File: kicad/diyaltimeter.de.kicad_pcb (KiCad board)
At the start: 2 copper layers, 45.7 x 97.8 mm, 12 parts, among them J1 Buttons, J2 Display, J3 links, J4 rechts, J5 I2C_BMP280, J6 I2C_BMP280_2, J7 RTC DS3231, J8 Conn_01x04_Male, SW1 SW_Push, SW2 SW_Push, SW3 SW_Push

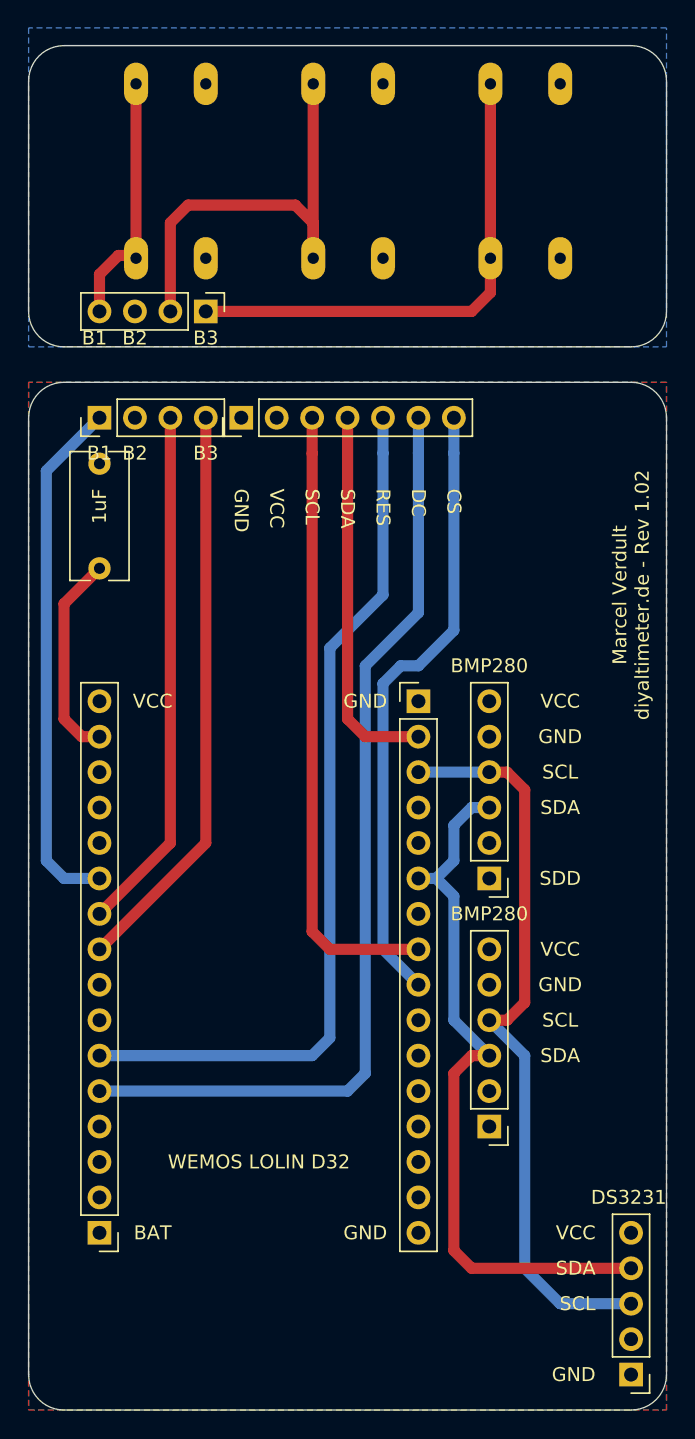
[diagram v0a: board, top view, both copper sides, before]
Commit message: final pcb
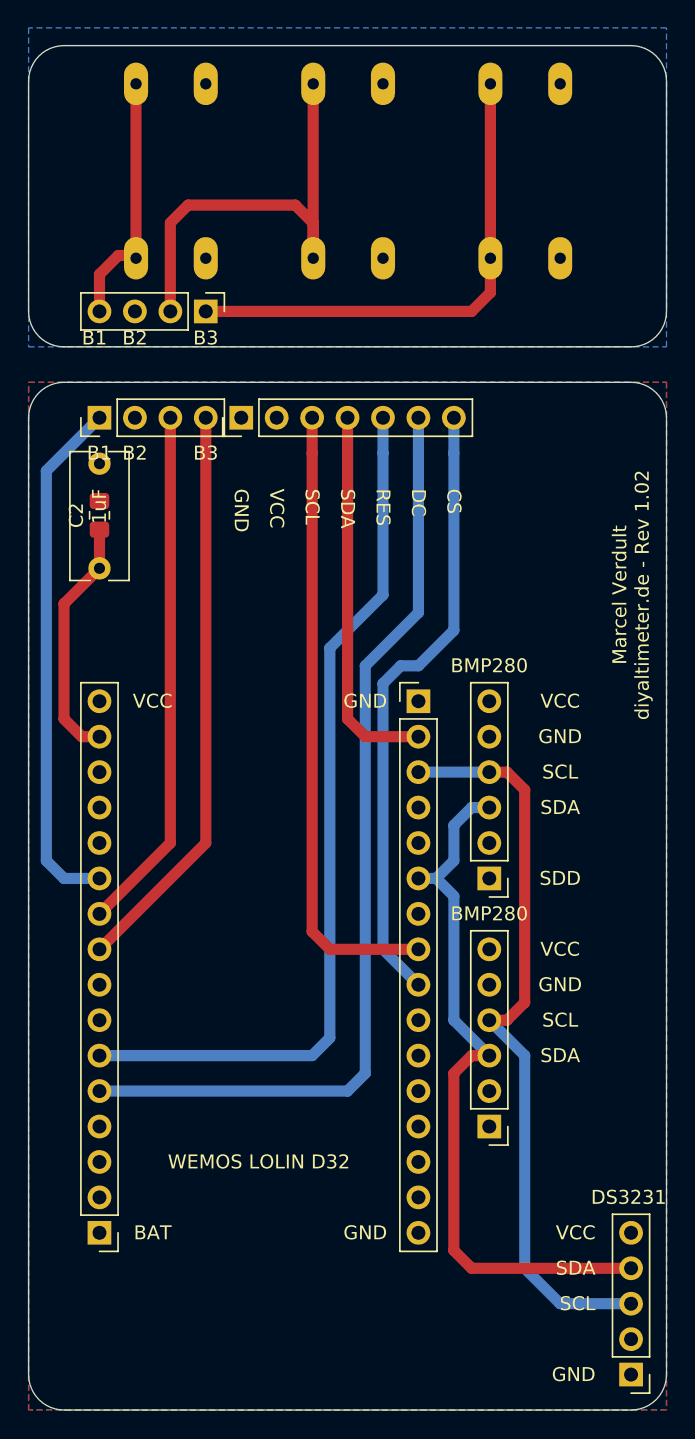
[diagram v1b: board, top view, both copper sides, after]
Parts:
- added C2: C, Capacitor_SMD:C_0805_2012Metric_Pad1.15x1.40mm_HandSolder, F.Cu at (71.1, 116.2)
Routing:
- net RS: track 14.9 -> 17.7 mm
